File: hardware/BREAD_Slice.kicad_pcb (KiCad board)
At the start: 2 copper layers, 72.6 x 100 mm, 16 parts, among them J1 Conn_01x10_Female, J2 I2C_01x04

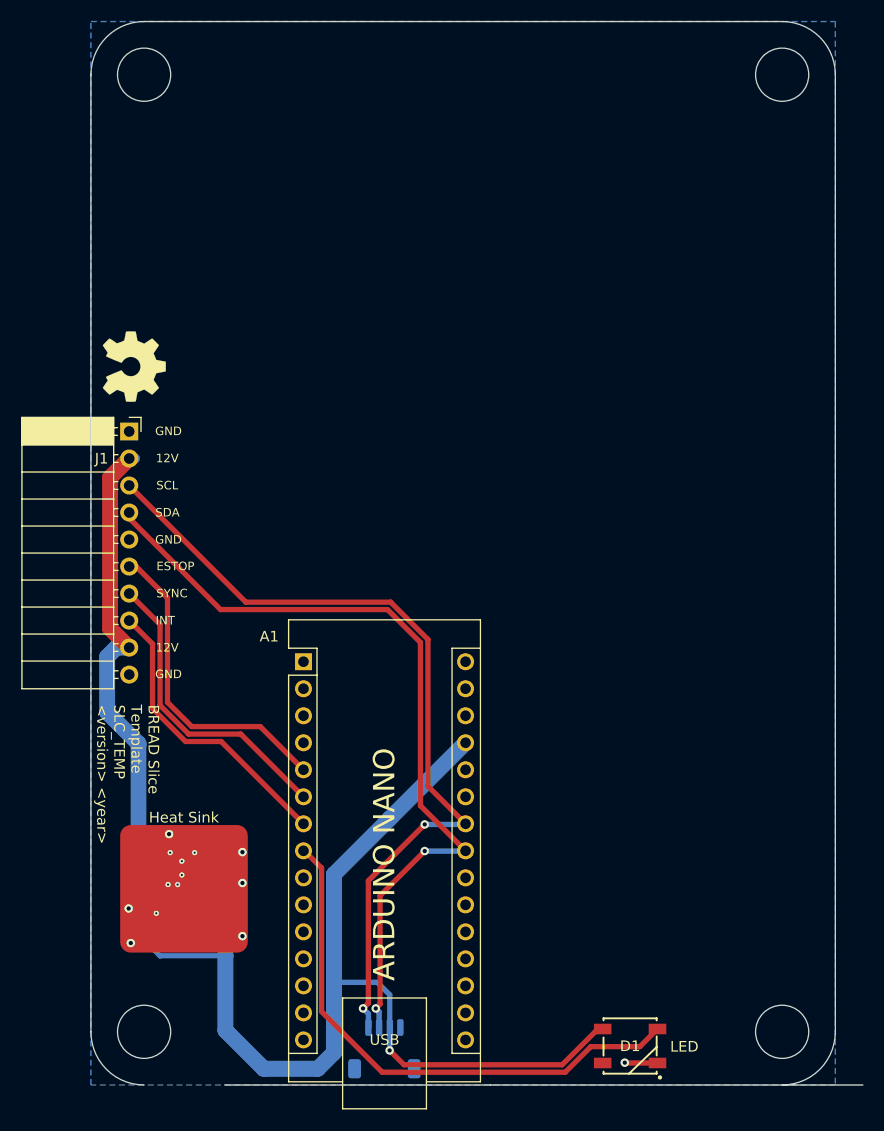
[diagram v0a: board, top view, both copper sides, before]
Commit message: Initial commit
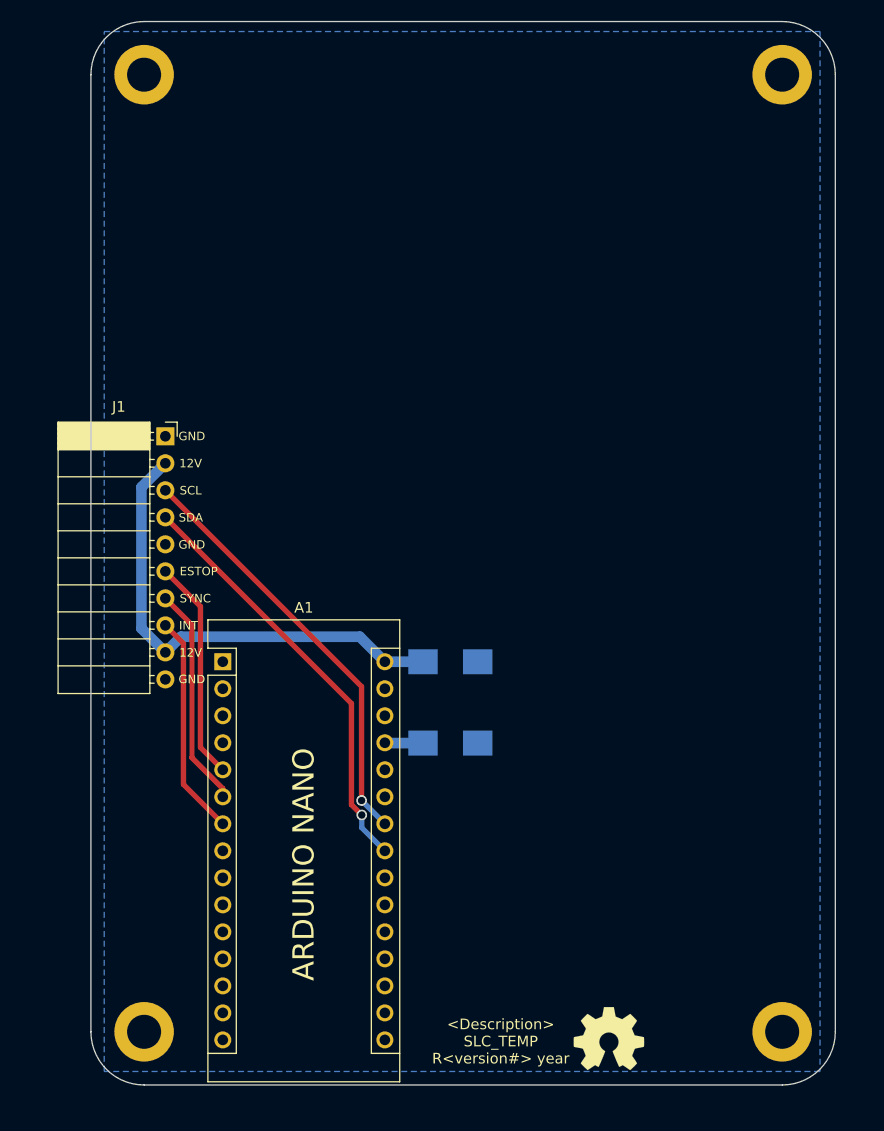
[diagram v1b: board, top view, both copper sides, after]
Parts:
- removed C3, C4: 22uF, Capacitor_SMD:C_1206_3216Metric
- removed D1: WS2812B_5050, SparkFun-LED:WS2812-5050-4PIN
- removed HS1: Heatsink_Pad, SparkFun-Fuse:Thermal Pad
- removed J2: I2C_01x04, Connector_JST:JST_SH_SM04B-SRSS-TB_1x04-1MP_P1.00mm_Horizontal
- removed L1: 4.7uH, Inductor_SMD:L_1210_3225Metric
- removed U1: ~, Package_TO_SOT_SMD:TSOT-23-6
- C1: value 22uF -> 10uF_t; footprint Capacitor_SMD:C_1206_3216Metric -> OCI_UPL_FOOTPRINTS:C_2312
- C2: value 100nF -> 10uF_t; footprint Capacitor_SMD:C_1206_3216Metric -> OCI_UPL_FOOTPRINTS:C_2312
- H1, H4: footprint MountingHole:MountingHole_5mm -> MountingHole:MountingHole_3.2mm_M3_DIN965_Pad
- H2: renamed from H3; footprint MountingHole:MountingHole_5mm -> MountingHole:MountingHole_3.2mm_M3_DIN965_Pad
- H3: renamed from H2; footprint MountingHole:MountingHole_5mm -> MountingHole:MountingHole_3.2mm_M3_DIN965_Pad
- moved Logo1 77.4 mm to (171.3, 135.4), turned to 0 degrees
- moved C1 34.0 mm to (156.4, 100.0), turned to 0 degrees
- moved C2 31.4 mm to (156.4, 107.7), turned to 0 degrees
- moved A1 7.59 mm to (135.0, 100.0)
- moved J1 3.43 mm to (129.6, 78.8)
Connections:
- A1 pad 10: unconnected-(A1-D7-Pad10) -> /BR2
- A1 pad 11: unconnected-(A1-D8-Pad11) -> /THRM2
- A1 pad 12: unconnected-(A1-D9-Pad12) -> /DIR1
- A1 pad 13: unconnected-(A1-D10-Pad13) -> /MC1
- A1 pad 14: unconnected-(A1-D11-Pad14) -> /BR1
- A1 pad 15: unconnected-(A1-D12-Pad15) -> /THRM1
- A1 pad 19: unconnected-(A1-A0-Pad19) -> /A1
- A1 pad 20: unconnected-(A1-A1-Pad20) -> /B1
- A1 pad 21: unconnected-(A1-A2-Pad21) -> /A2
- A1 pad 22: unconnected-(A1-A3-Pad22) -> /B2
- A1 pad 25: unconnected-(A1-A6-Pad25) -> /CSEN1
- A1 pad 26: unconnected-(A1-A7-Pad26) -> /CSEN2
- A1 pad 30: unconnected-(A1-VIN-Pad30) -> +12V
- A1 pad 8: /LED -> /DIR2
- A1 pad 9: unconnected-(A1-D6-Pad9) -> /MC2
- C1 pad 1: GND -> +12V
- C1 pad 2: +12V -> GND
- C2 pad 1: Net-(U1-SW) -> +5V
- C2 pad 2: Net-(U1-BST) -> GND
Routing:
- net +5V: track 108.9 -> 3.60 mm, vias 1 -> 0
- net /LED: track 51.5 -> 0.00 mm
- net /I2C_CLK: track 78.5 -> 39.9 mm, vias 2 -> 1
- net /I2C_DAT: track 76.6 -> 39.9 mm, vias 2 -> 1
- net GND: track 19.6 -> 0.00 mm, vias 14 -> 0
- net /E_STOP: track 30.1 -> 20.9 mm
- net /INT: track 28.8 -> 20.9 mm
- net /SYNC: track 27.9 -> 20.9 mm
- net Net-(U1-SW): track 5.22 -> 0.00 mm
- net Net-(U1-BST): track 2.64 -> 0.00 mm
- net +12V: track 46.8 -> 45.5 mm
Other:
- board size 72.6 x 100 mm -> 70 x 100 mm
- board text added: "<Description> SLC_TEMP R<version#> year"
- board text removed: "12V->5V Reg"
- board text removed: "5V I2C Connector"
- board text removed: "BREAD Slice Template SLC_TEMP <version> <year>"
- board text removed: "LED"
